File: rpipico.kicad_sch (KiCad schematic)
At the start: 36 parts, among them J1 USB_C_Receptacle_USB2.0, J2 Conn_01x02_Pin, J3 Conn_01x13, J4 Conn_01x13, J5 Conn_01x04, J6 Conn_01x03, J7 Conn_01x04, J8 Conn_01x02, J9 Conn_01x02, U2 W25Q128JVS, U3 RP2040, U5 AP2112K-3.3, Y1 12M

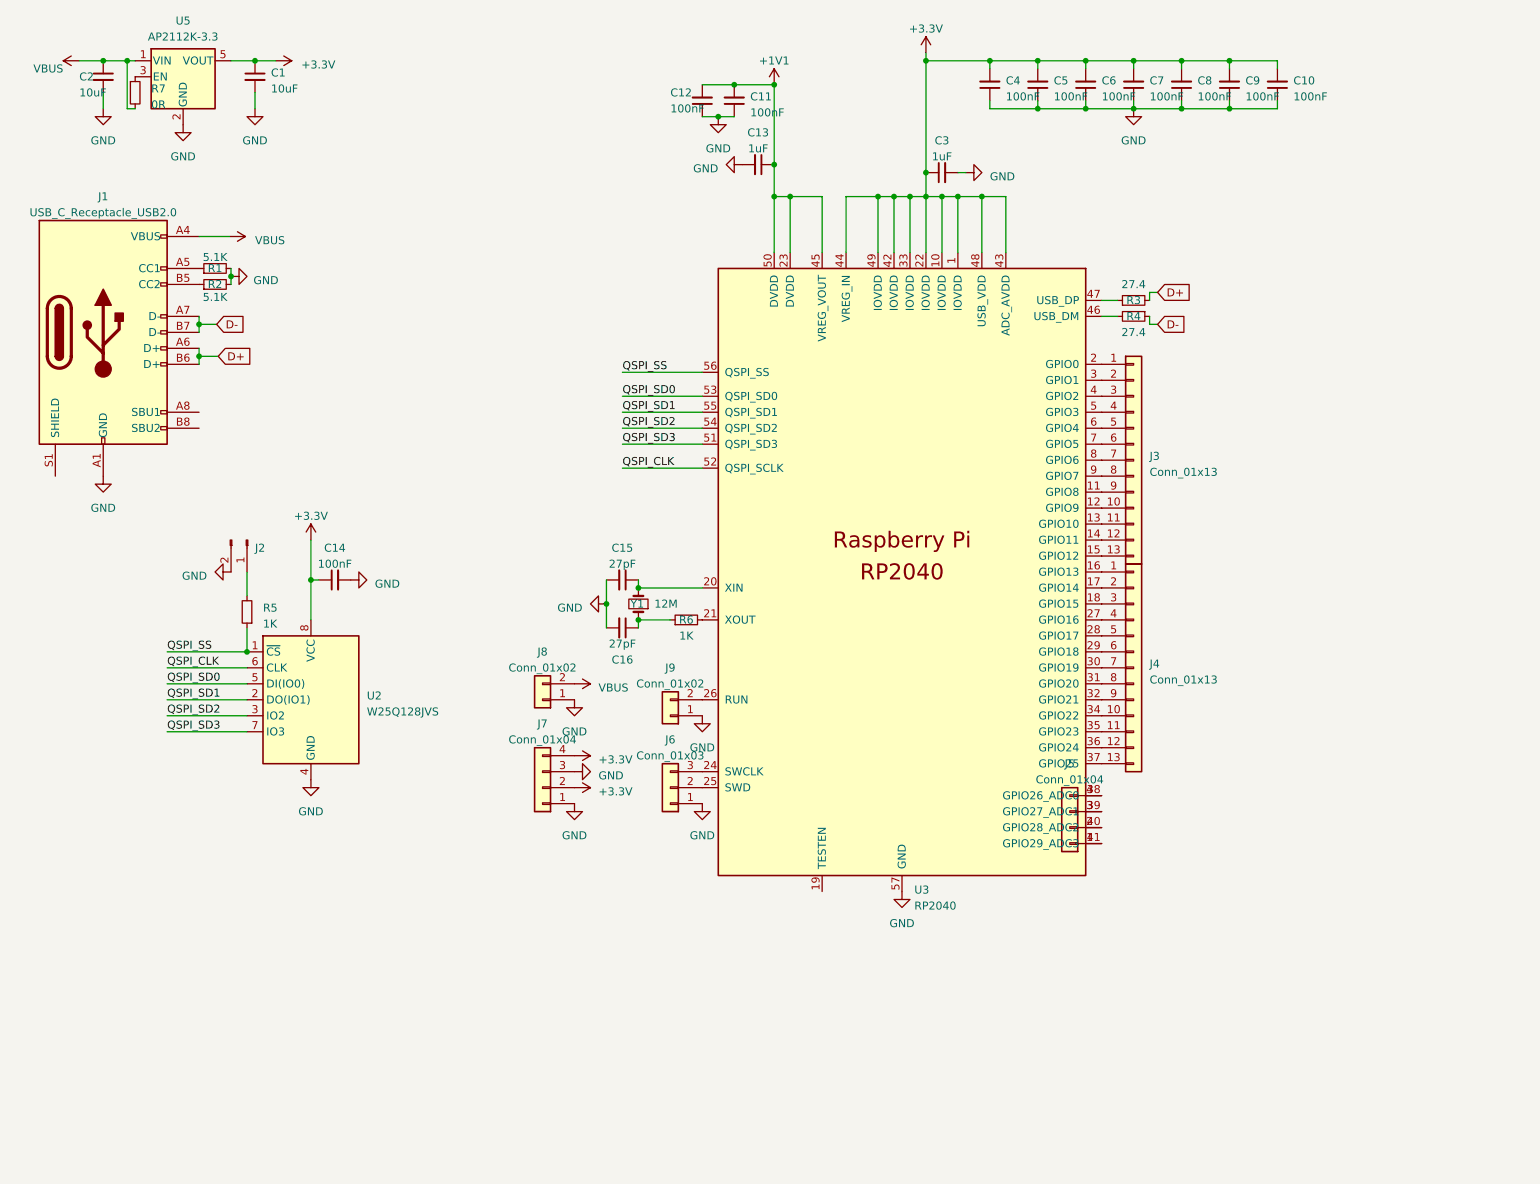
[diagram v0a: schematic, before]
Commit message: Add files via upload
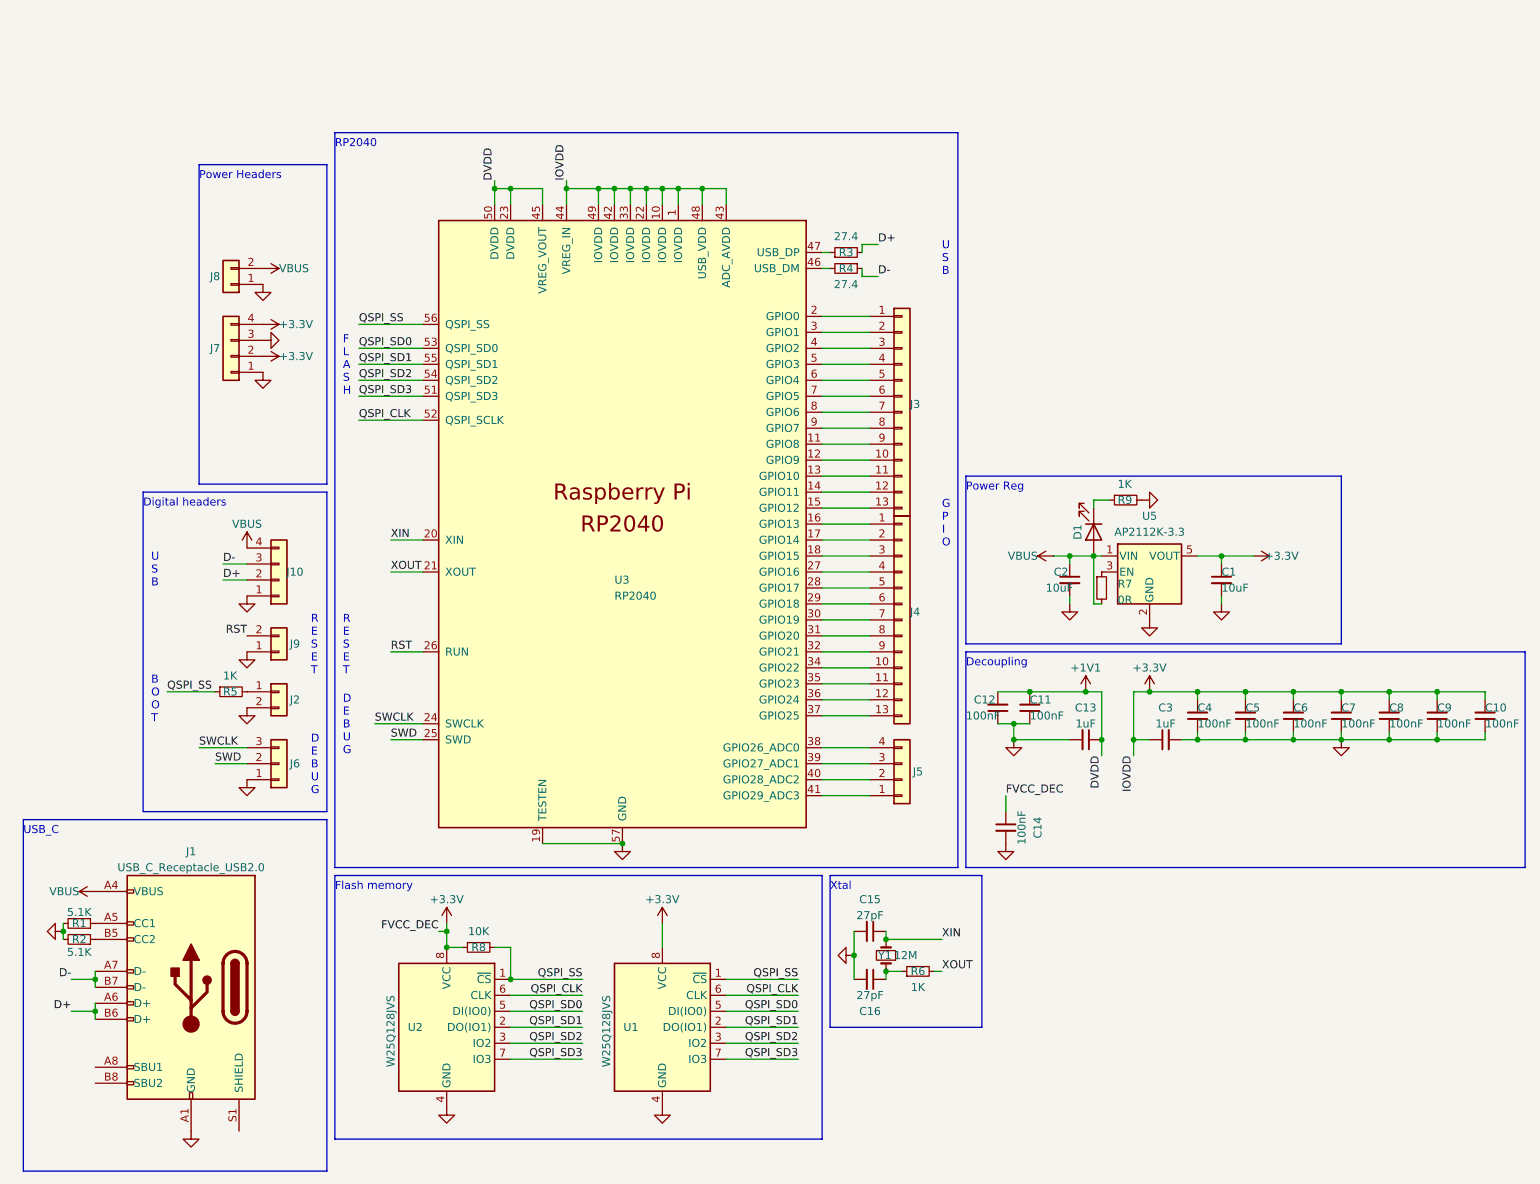
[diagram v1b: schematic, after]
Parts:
- removed J2: Conn_01x02_Pin, Connector_PinHeader_1.00mm:PinHeader_1x02_P1.00mm_Vertical, symbol Connector:Conn_01x02_Pin
- added D1: LED, LED_SMD:LED_0603_1608Metric, symbol Device:LED
- added J10: Conn_01x04, Connector_PinHeader_1.00mm:PinHeader_1x04_P1.00mm_Vertical, symbol Connector_Generic:Conn_01x04
- added J2: Conn_01x02, Connector_PinHeader_1.00mm:PinHeader_1x02_P1.00mm_Vertical, symbol Connector_Generic:Conn_01x02
- added R8: 10K, Resistor_SMD:R_0402_1005Metric, symbol Device:R_Small
- added R9: 1K, Resistor_SMD:R_0402_1005Metric, symbol Device:R_Small
- added U1: W25Q128JVS, Package_DFN_QFN:DFN-8-1EP_3x2mm_P0.5mm_EP1.3x1.5mm, symbol Memory_Flash:W25Q128JVS
- R6: footprint Resistor_SMD:R_0402_1005Metric -> Resistor_SMD:R_0201_0603Metric
- Y1: footprint Crystal2:Crystal_2.0mm_2.5mm -> Crystal:Crystal_SMD_3225-4Pin_3.2x2.5mm
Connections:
- net +3.3V: now also R8.1, U1.8 (VCC)
- net D+: now also J10.2 (Pin_2)
- net D-: now also J10.3 (Pin_3)
- net GND: now also U3.19 (TESTEN), J10.1 (Pin_1), J2.2 (Pin_2), R9.2, U1.4 (GND)
- net QSPI_CLK: now also U1.6 (CLK)
- net QSPI_SD0: now also U1.5 (DI(IO0))
- net QSPI_SD1: now also U1.2 (DO(IO1))
- net QSPI_SD2: now also U1.3 (IO2)
- net QSPI_SD3: now also U1.7 (IO3)
- net QSPI_SS: now also R8.2, U1.1 (~{CS})
- net VBUS: now also D1.2 (A), J10.4 (Pin_4)
- net at R5.2: now also J2.1 (Pin_1)
- net XIN: now reaches C15.1, U3.20 (XIN), Y1.2
- net XOUT: now reaches R6.2, U3.21 (XOUT)
- net SWCLK: now reaches J6.3 (Pin_3), U3.24 (SWCLK)
- net SWD: now reaches J6.2 (Pin_2), U3.25 (SWD)
- net RST: now reaches J9.2 (Pin_2), U3.26 (RUN)
- new net: D1.1 (K), R9.1
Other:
- note added: "B O O T"
- note added: "D E B U G"
- note added: "Decoupling"
- note added: "Digital headers"
- note added: "F L A S H"
- note added: "Flash memory"
- note added: "G P I O"
- note added: "Power Headers"
- note added: "Power Reg"
- note added: "R E S E T"
- note added: "RP2040"
- note added: "U S B"
- note added: "USB_C"
- note added: "Xtal"
- moved on the sheet: C1, C10, C11, C12, C13, C14, C15, C16, C2, C3, C4, C5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
